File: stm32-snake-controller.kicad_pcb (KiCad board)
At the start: 4 copper layers, 162.5 x 72 mm, 62 parts, among them J101 Barrel_Jack_MountingPin, J102 JST 2.54 Header, J103 Tag Connector, J301 Conn_01x03, J302 Conn_01x03, J401 Conn_01x07, J402 Conn_01x07, J501 USB_A, Q101 AO3501A, SW101 SW_Push, SW102 SW_Push, SW301 SW_SPDT, U101 USBLC6-2SC6, U102 M24C64-RMN, U103 STM32F401RCTx, U201 XC6220B331MR-G, U301 74AHCT1G125, U302 74AHCT1G125, U501 STMPS2141STR, Y101 32.768kHz, Y102 16MHz

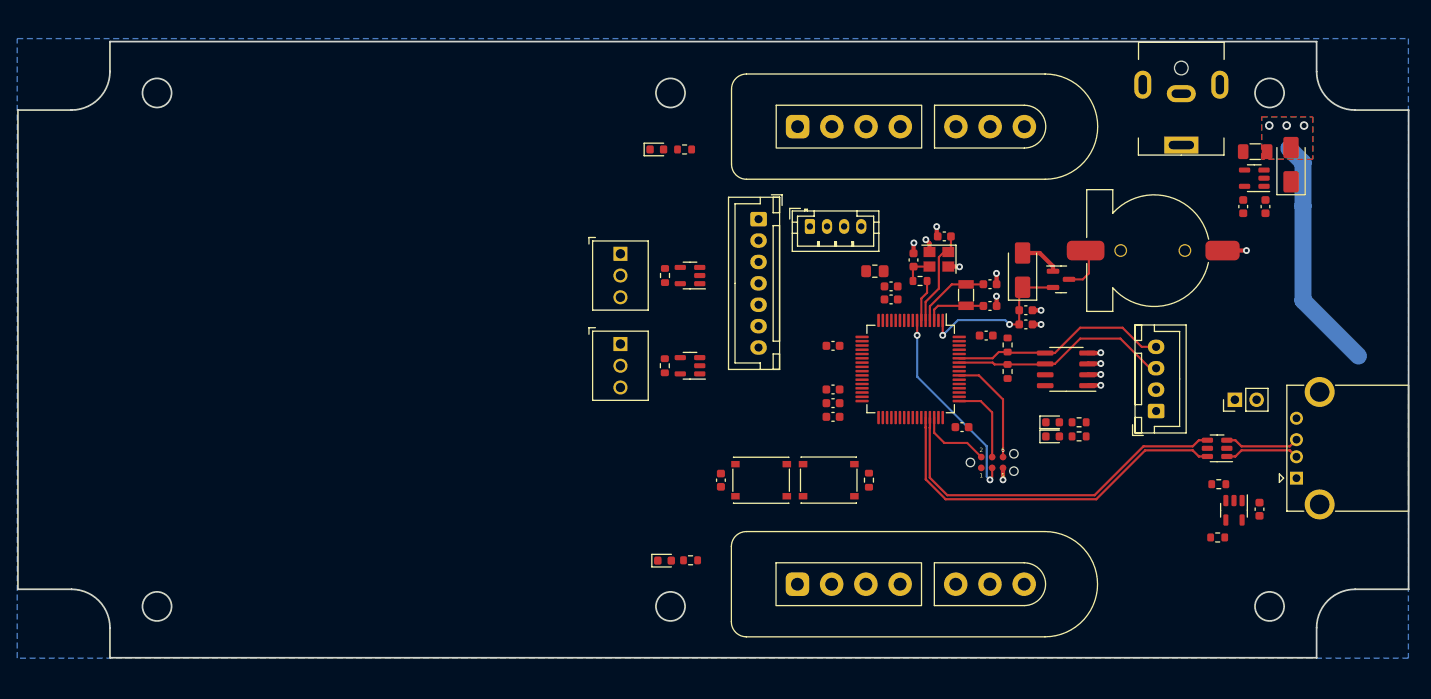
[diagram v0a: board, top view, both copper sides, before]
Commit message: update PCB design
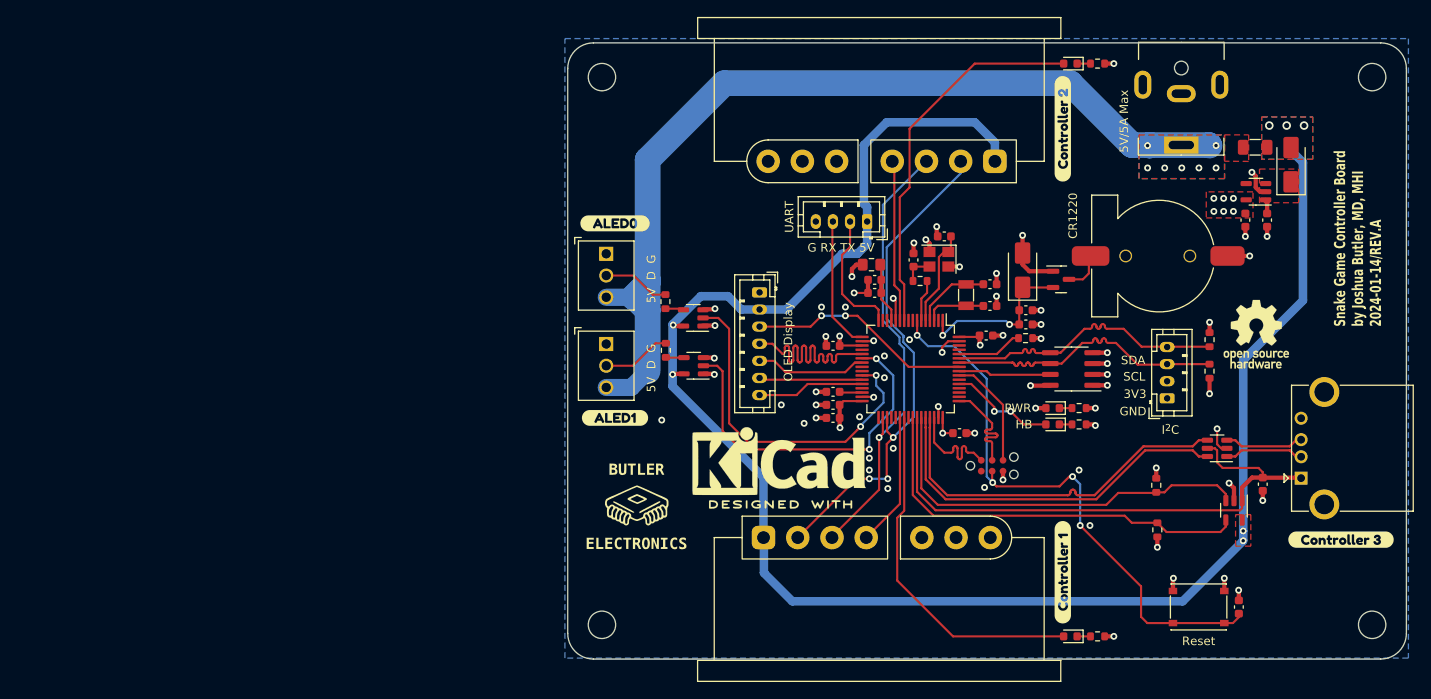
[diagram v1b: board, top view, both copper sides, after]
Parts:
- removed the R101 at (174.2, 115.1)
- removed SW102: SW_Push, User_Footprint:XKB-Connectivity-TS-1187A-B-A-B
- removed SW301: SW_SPDT, Connector_PinHeader_2.54mm:PinHeader_1x02_P2.54mm_Vertical
- added G***: LOGO, User_Footprint:butler-electronics-15, F.Cu at (147.1, 118.1)
- added H101: MountingHole, MountingHole:MountingHole_3.2mm_M3, F.Cu at (143.0, 68.0)
- added H102: MountingHole, MountingHole:MountingHole_3.2mm_M3, F.Cu at (233.0, 68.0)
- added H103: MountingHole, MountingHole:MountingHole_3.2mm_M3, F.Cu at (233.0, 132.0)
- added H104: MountingHole, MountingHole:MountingHole_3.2mm_M3, F.Cu at (143.0, 132.0)
- added R102: 10K, Resistor_SMD:R_0603_1608Metric, F.Cu at (192.5, 98.5)
- added REF**: KiCad-Logo2_8mm_SilkScreen, Symbol:KiCad-Logo2_8mm_SilkScreen, F.Cu at (163.7, 112.8)
- added REF**: OSHW-Logo_7.5x8mm_SilkScreen, Symbol:OSHW-Logo_7.5x8mm_SilkScreen, F.Cu at (219.5, 98.0)
- added kibuzzard-65A37CF1: G***, kibuzzard-65A37CF1, F.Cu at (196.8, 74.0)
- added kibuzzard-65A37D11: G***, kibuzzard-65A37D11, F.Cu at (196.8, 125.9)
- added kibuzzard-65A37DD1: G***, kibuzzard-65A37DD1, F.Cu at (229.4, 122.0)
- added kibuzzard-65A37F11: G***, kibuzzard-65A37F11, F.Cu at (144.5, 85.1)
- added kibuzzard-65A37F1A: G***, kibuzzard-65A37F1A, F.Cu at (144.5, 107.8)
- J401, J402: footprint User_Footprint:SNES_Controller_Port -> User_Footprint:SNES_Controller_Port_Horizontal
- OLED101: renamed from OLED102; footprint Connector_JST:JST_XH_B4B-XH-A_1x04_P2.50mm_Vertical -> Connector_JST:JST_PH_B4B-PH-K_1x04_P2.00mm_Vertical
- OLED102: renamed from OLED101; footprint Connector_JST:JST_XH_B7B-XH-A_1x07_P2.50mm_Vertical -> Connector_JST:JST_PH_B7B-PH-K_1x07_P2.00mm_Vertical
- moved R103 75.0 mm to (200.9, 66.4)
- moved D104 75.0 mm to (197.7, 66.4), turned to 180 degrees
- moved D105 74.6 mm to (197.7, 133.3), turned to 180 degrees
- moved R104 74.6 mm to (200.9, 133.3)
- moved C110 62.3 mm to (217.4, 129.9), turned to 90 degrees
- moved SW101 53.2 mm to (212.7, 129.9), turned to 180 degrees
- moved J402 49.6 mm to (175.3, 77.8), turned to 180 degrees
- moved J401 48.2 mm to (175.5, 121.8)
- moved R107 23.6 mm to (214.0, 98.7)
- moved R108 23.6 mm to (214.0, 102.4)
- moved OLED102 8.56 mm to (161.4, 93.2)
- moved R501 7.30 mm to (207.8, 115.7), turned to 90 degrees
- moved R502 7.10 mm to (207.9, 120.9), turned to -90 degrees
- moved J102 6.71 mm to (174.0, 84.9), turned to 180 degrees
- moved U301 4.97 mm to (153.7, 96.1)
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- renumbered C114 to C101, C115 to C102, C106 to C103, C108 to C104, C110 to C105, C111 to C106, C113 to C107, C107 to C108, C103 to C110, C101 to C111, C104 to C112, C105 to C113, C102 to C114, C112 to C115, D106 to D102, D102 to D103, D103 to D104, D104 to D105, D105 to D106, R104 to R101, R105 to R103, R106 to R104, R107 to R105, R102 to R106, R103 to R107, R502 to R501, R501 to R502
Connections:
- D104 pad 2: /LED_SNES0 -> /LED_SNES1
- D105 pad 2: /LED_SNES1 -> /LED_SNES0
- J301 pad 3: /LED_PWR -> VBUS
- J302 pad 3: /LED_PWR -> VBUS
- OLED102 pad 2: +3V3 -> +5V
- OLED102 pad 3: /SPI_CLK -> /MOSI
- OLED102 pad 4: /MOSI -> /SPI_CLK
- OLED102 pad 6: /OLED_DC -> /OLED_CE
- OLED102 pad 7: /OLED_CE -> /OLED_DC
- U101 pad 5: VBUS -> /USB_OTG_VSEN
- U103 pad 10: unconnected-(U103-PC2-Pad10) -> /LED_SNES1
- U103 pad 11: unconnected-(U103-PC3-Pad11) -> /SNES_DATA1
- U103 pad 24: /LED_SNES0 -> unconnected-(U103-PC4-Pad24)
- U103 pad 25: /LED_SNES1 -> unconnected-(U103-PC5-Pad25)
- U103 pad 33: /~{EEPROM} -> unconnected-(U103-PB12-Pad33)
- U103 pad 37: /SNES_DATA1 -> unconnected-(U103-PC6-Pad37)
- U103 pad 39: unconnected-(U103-PC8-Pad39) -> /LED_SNES0
- U103 pad 56: unconnected-(U103-PB4-Pad56) -> /~{EEPROM}
- U103 pad 60: /BOOT0 -> Net-(U103-BOOT0)
- U301 pad 2: /LED_GRID0 -> /LED_GRID1
- U302 pad 2: /LED_GRID1 -> /LED_GRID0
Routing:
- net +5V: track 0.00 -> 205.0 mm, vias 3 -> 7
- net VBUS: track 0.00 -> 111.1 mm, vias 0 -> 7
- net /USB_OTG_VSEN: track 0.00 -> 66.5 mm
- net /SNES_CLK: track 0.00 -> 59.4 mm, vias 0 -> 3
- net /SNES_LATCH: track 0.00 -> 53.1 mm, vias 0 -> 1
- net /USB_OTG_EN: track 0.00 -> 48.5 mm
- net GND: track 20.2 -> 67.1 mm, vias 14 -> 60
- net /USB_OTG_OC: track 0.00 -> 46.8 mm
- net /LED_SNES1: track 0.00 -> 44.2 mm
- net /NRST: track 23.7 -> 67.9 mm, vias 2 -> 4
- net /LED_GRID0: track 0.00 -> 41.8 mm, vias 0 -> 2
- net /LED_SNES0: track 0.00 -> 41.5 mm
- net /LED_GRID1: track 0.00 -> 40.7 mm, vias 0 -> 2
- net +3V3: track 4.77 -> 34.5 mm, vias 0 -> 18
- net /SPI_CLK: track 0.00 -> 29.2 mm
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- added copper zone on F.Cu, net +3V3
- added copper zone on F.Cu, net /LDO_3V3/5V
- added copper zone on B.Cu, net VBUS
- added copper zone on F.Cu, net VBUS
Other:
- board size 162.5 x 72 mm -> 98 x 72 mm
- board text added: "${TITLE} by ${COMMENT1} ${ISSUE_DATE}/REV.${REVISION}"
- board text added: "3V3"
- board text added: "5V D G"
- board text added: "5V/5A Max"
- board text added: "CR1220"
- board text added: "G RX TX 5V"
- board text added: "GND"
- board text added: "HB"
- board text added: "I^{2}C"
- board text added: "JLCJLCJLCJLC"
- board text added: "OLED Display"
- board text added: "PWR"
- board text added: "Reset"
- board text added: "SCL"
- board text added: "SDA"
- board text added: "UART"
